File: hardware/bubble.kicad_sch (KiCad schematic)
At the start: 41 parts, among them Q1 BS170, U1 i7254, U2 i7250, U3 74LS74, U4 i7254, U5 i7230, U6 i7220, U7 i7242, Y1 8.000 MHz

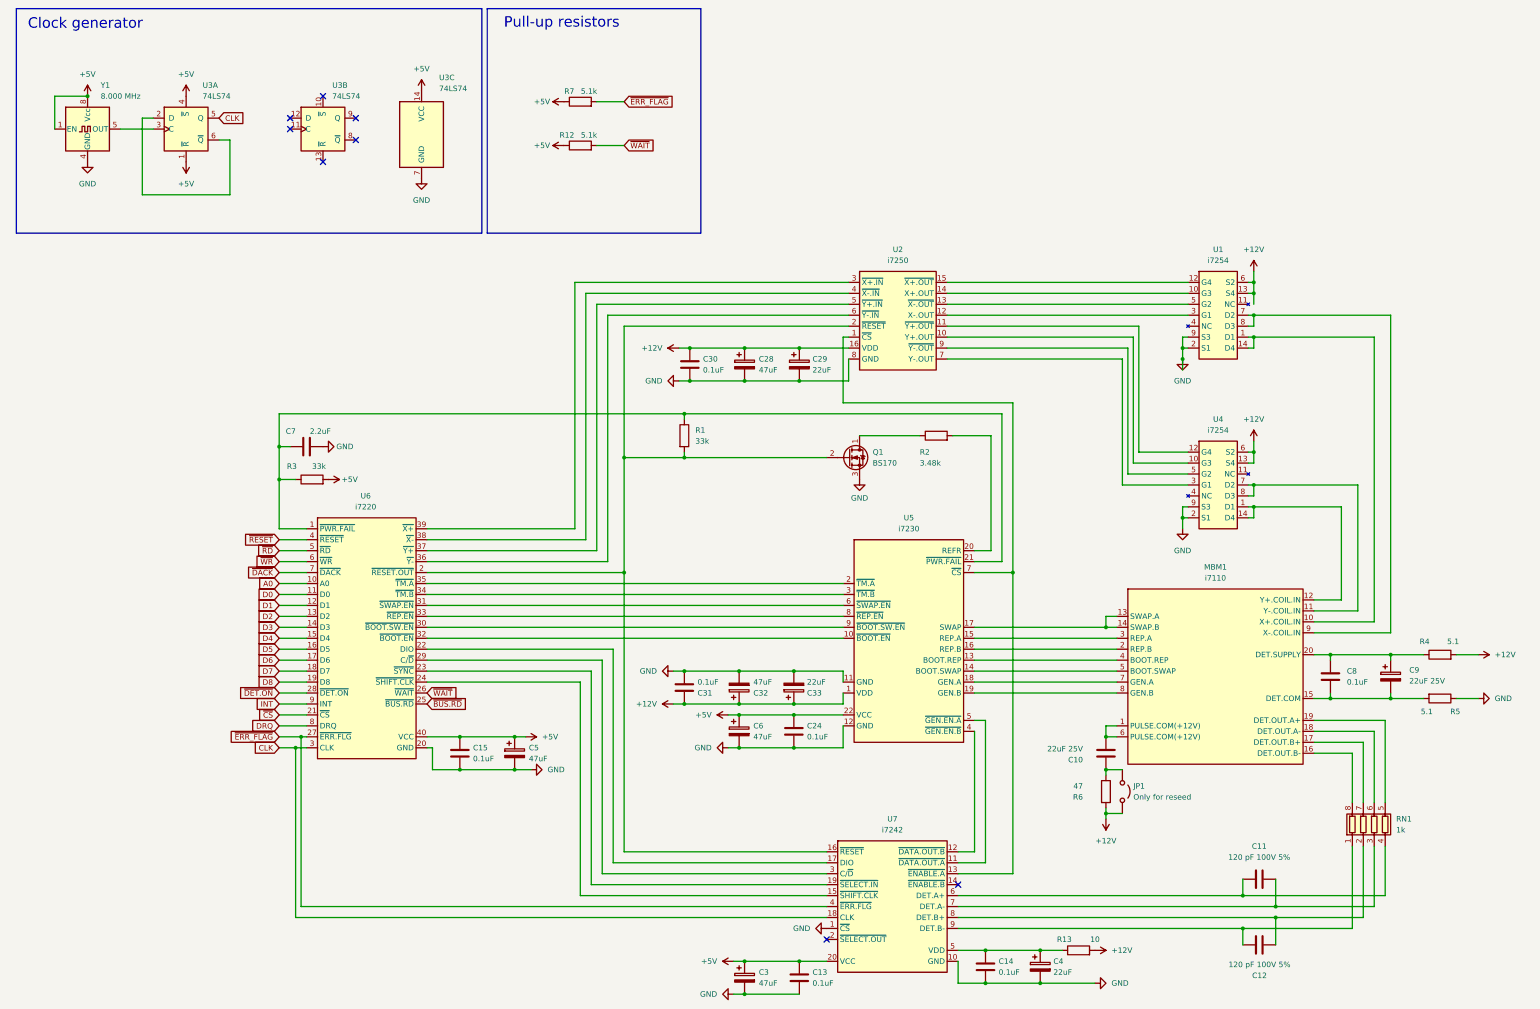
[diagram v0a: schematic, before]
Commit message: hardware: minor cleanup
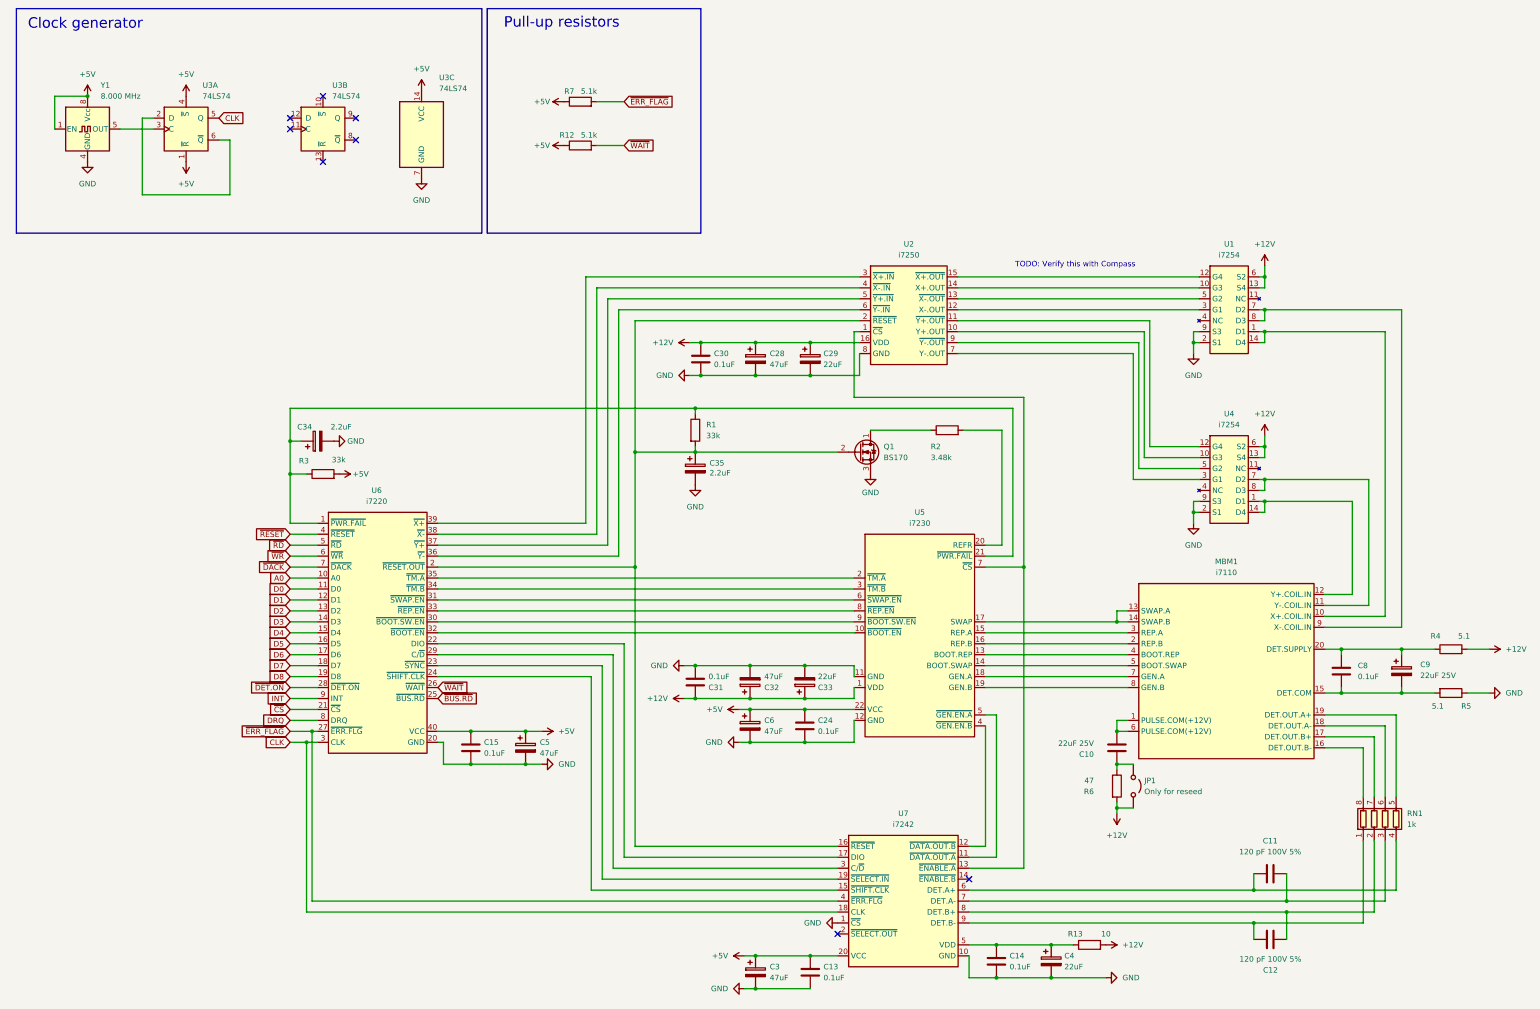
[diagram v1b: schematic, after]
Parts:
- removed C7: 2.2uF, Capacitor_THT:C_Radial_D4.0mm_H7.0mm_P1.50mm, symbol Device:C
- added C34, C35: 2.2uF, Capacitor_THT:CP_Radial_D5.0mm_P2.00mm, symbol Device:C_Polarized
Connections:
- net GND: now also C34.2, C35.2
- net at R1.1, R3.1, U5.21 (~{PWR.FAIL})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: now also C34.1
- net at Q1.2 (G), R1.2, U2.2 (~{RESET})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: now also C35.1
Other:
- note added: "TODO: Verify this with Compass"
- moved on the sheet: C10, C11, C12, C13, C14, C15, C24, C28, C29, C3, C30, C31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
